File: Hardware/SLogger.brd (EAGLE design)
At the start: 22 x 33.5 mm, 16 parts, among them U2 DSPIC33FJ802GP-28, U7 USD-SOCKETNEW

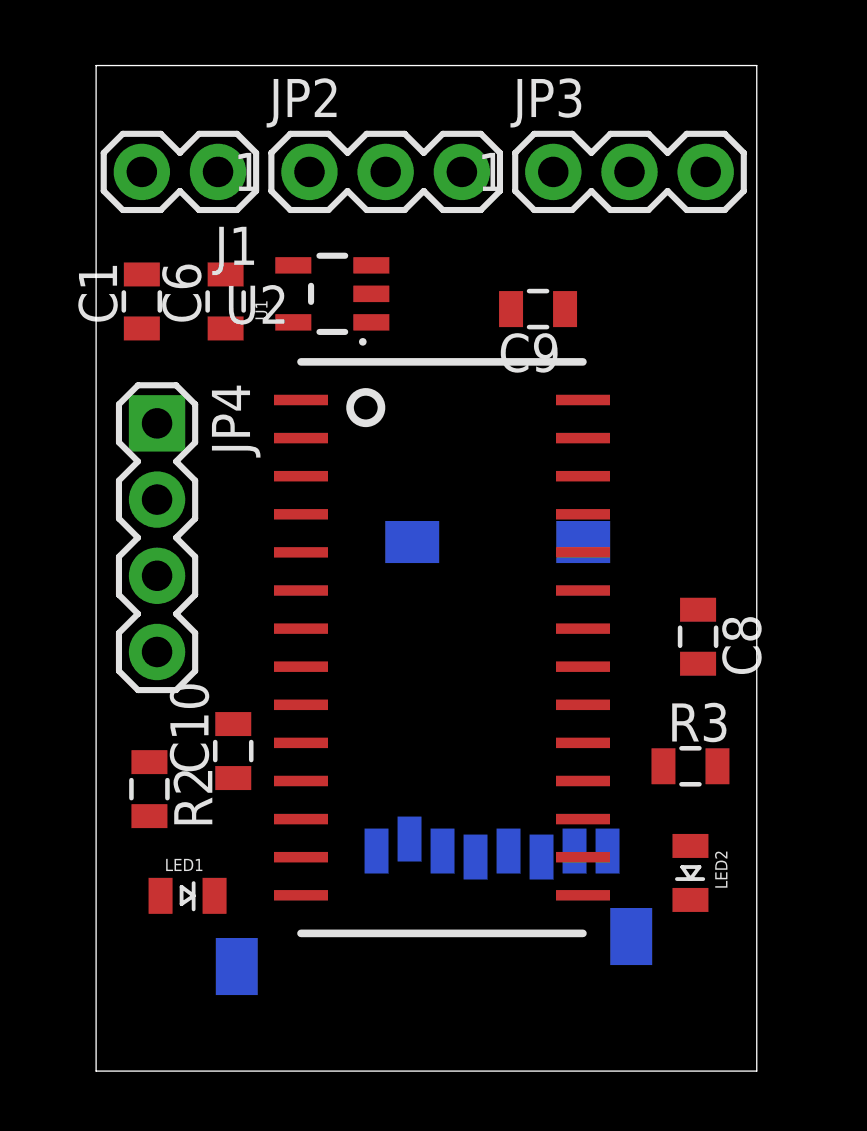
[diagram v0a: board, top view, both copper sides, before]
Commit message: Finished 1.0 version of the new SLogger hardware.
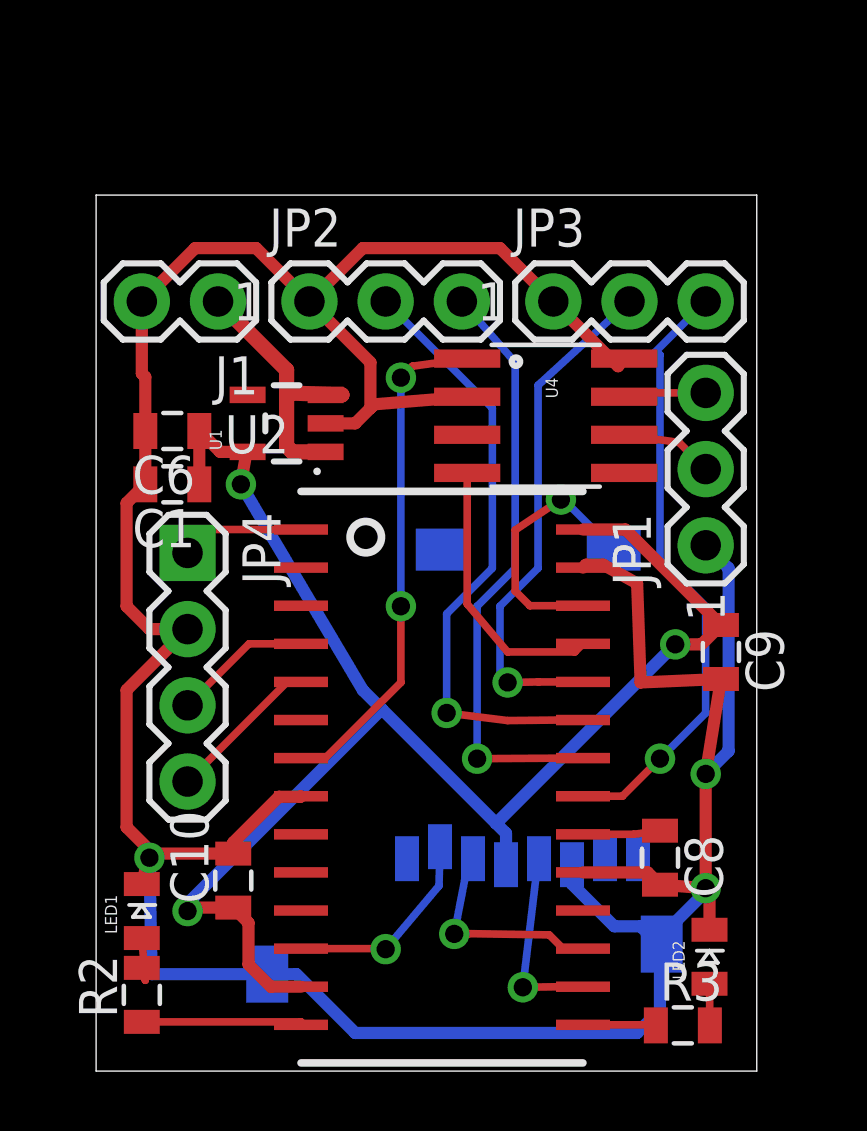
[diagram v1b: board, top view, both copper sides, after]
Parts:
- added JP1: M03PTH, ASL:1X03
- added U4: MCP2551, SparkFun:SO08
- moved C9 13.0 mm to (20.8, 14.0), turned to 270 degrees
- moved R3 8.64 mm to (19.6, 1.52)
- moved C8 7.47 mm to (18.8, 7.11)
- moved R2 6.86 mm to (1.52, 2.54), turned to 90 degrees
- moved C1 6.18 mm to (2.54, 19.6), turned to 180 degrees
- moved C6 4.67 mm to (2.54, 21.3), turned to 180 degrees
- moved U1 4.58 mm to (6.35, 21.6)
- moved JP4 4.44 mm to (3.05, 17.3)
- moved J1 4.32 mm to (4.06, 25.7)
- moved JP2 4.32 mm to (9.65, 25.7)
- moved JP3 4.32 mm to (17.8, 25.7)
- moved U2 4.32 mm to (11.4, 9.65)
- moved C10 4.32 mm to (4.57, 6.35)
- moved LED2 2.87 mm to (20.4, 3.81), turned to 90 degrees
- moved LED1 1.61 mm to (1.52, 5.33), turned to 90 degrees
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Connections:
- new net CAN_HI: JP1.3, U4.7
- new net CAN_LO: JP1.2, U4.6
- new net CAN_RX: U2.P$25, U4.4
- new net CAN_TX: U2.P$7, U4.1
- new net VCC5V0: U4.3
- net GND: now also JP1.1, U4.2, U4.8
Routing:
- net GND: track 0.00 -> 120.1 mm, vias 0 -> 3
- net VCC3V3: track 0.00 -> 51.8 mm, vias 0 -> 3
- net UART2_TX: track 0.00 -> 20.6 mm, vias 0 -> 1
- net UART1_RX: track 0.00 -> 20.4 mm, vias 0 -> 1
- net UART1_TX: track 0.00 -> 20.0 mm, vias 0 -> 1
- net UART2_RX: track 0.00 -> 17.2 mm, vias 0 -> 1
- net CAN_TX: track 0.00 -> 16.9 mm, vias 0 -> 2
- net VCC: track 0.00 -> 9.54 mm
- net CAN_RX: track 0.00 -> 9.09 mm
- net CD: track 0.00 -> 8.91 mm, vias 0 -> 1
- net SDO: track 0.00 -> 7.32 mm, vias 0 -> 1
- net CS: track 0.00 -> 6.93 mm, vias 0 -> 1
- net SCK: track 0.00 -> 6.34 mm, vias 0 -> 1
- net PGC: track 0.00 -> 6.23 mm
- net LED1: track 0.00 -> 5.40 mm
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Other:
- board size 22 x 33.5 mm -> 22 x 29.2 mm
